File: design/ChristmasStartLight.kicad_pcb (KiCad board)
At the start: 2 copper layers, 12.5 x 25.8 mm, 8 parts, among them P101 CONN_01X02, Q101 MMBT3904-7-F, SW101 MHSS1104, U101 ICM7555CBAZ-T

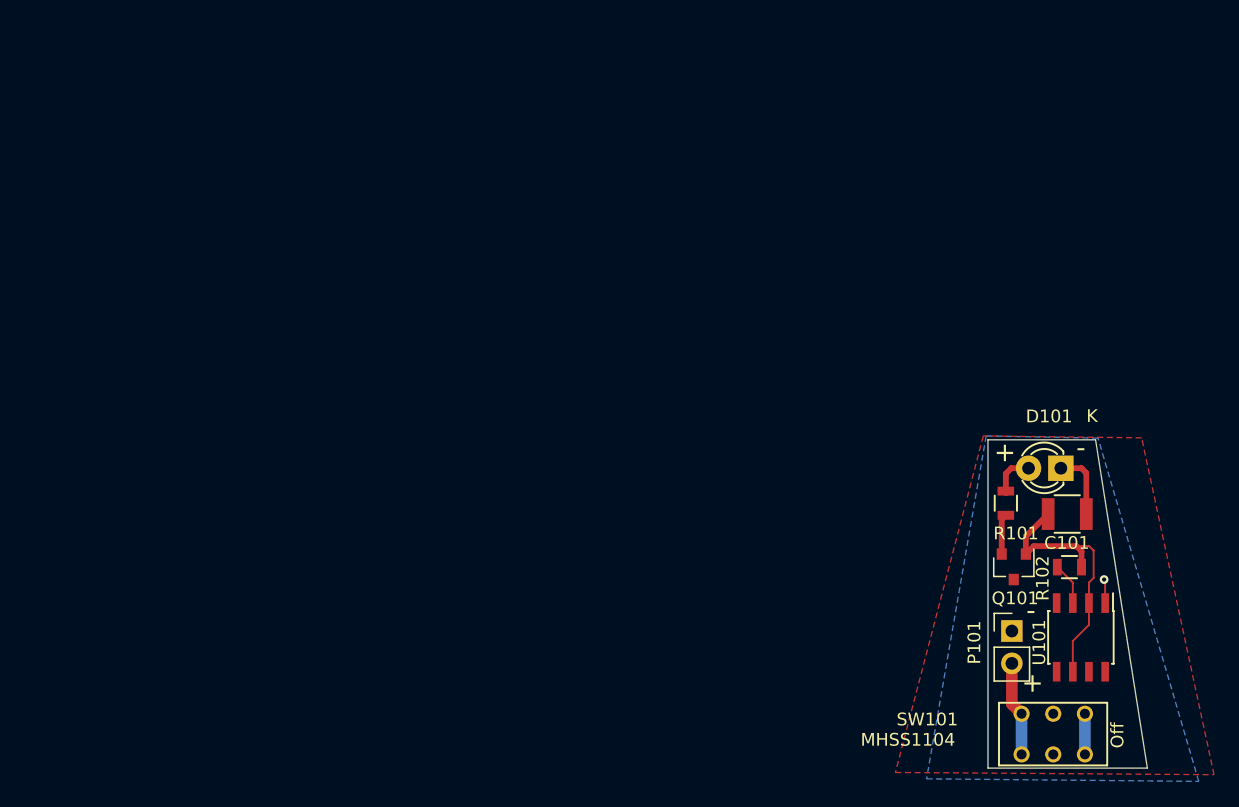
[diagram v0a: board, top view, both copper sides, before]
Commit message: Misc changes
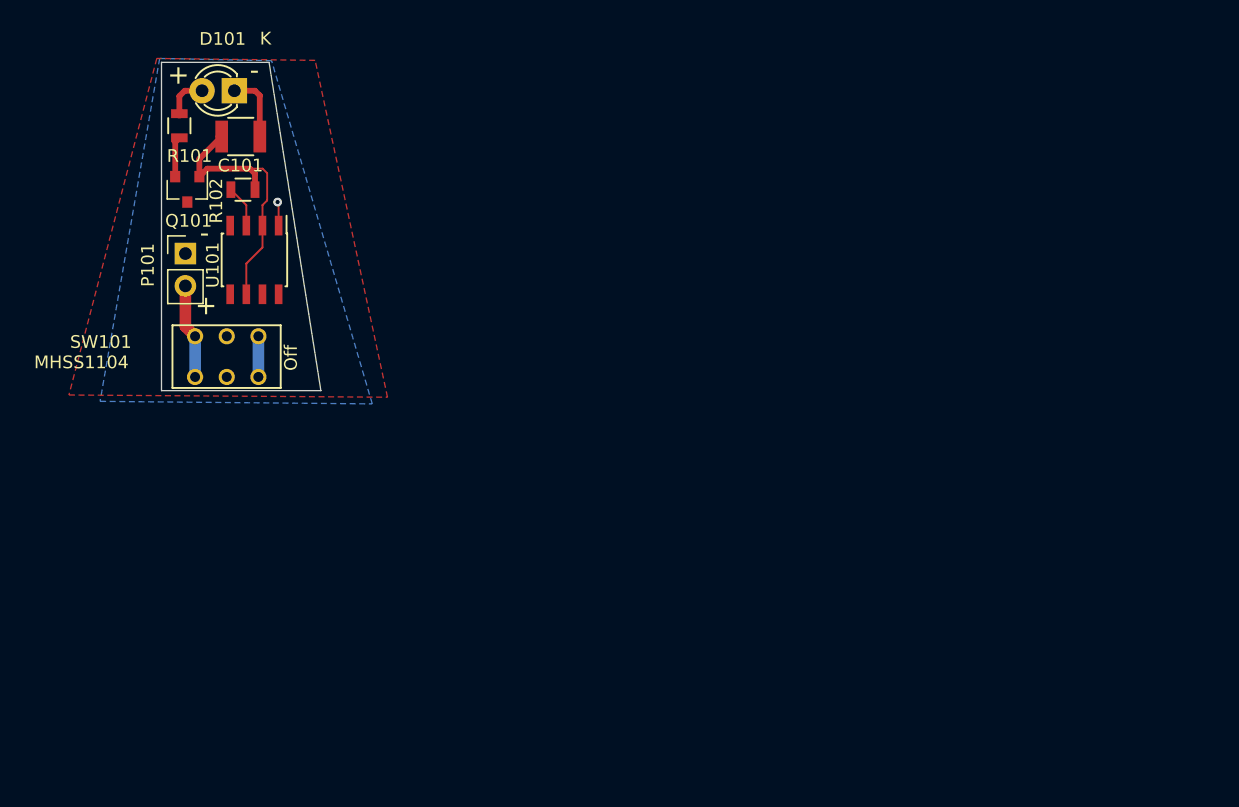
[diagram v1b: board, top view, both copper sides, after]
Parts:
- moved C101 71.4 mm to (64.8, 28.9)
- moved D101 71.4 mm to (64.3, 25.2)
- moved R102 71.4 mm to (65.0, 33.0)
- moved SW101 71.4 mm to (63.6, 46.1)
- moved P101 71.4 mm to (60.5, 38.0)
- moved Q101 71.4 mm to (60.6, 33.0)
- moved R101 71.4 mm to (60.0, 28.0)
- moved U101 71.4 mm to (65.9, 38.5)
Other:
- board text removed: "1.9.2017"
- board text removed: "v2"
